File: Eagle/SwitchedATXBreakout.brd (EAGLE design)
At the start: 101.3 x 80 mm, 47 parts, among them K1 ALF1P05, K2 ALF1P05, K3 ALF1P05, K4 ALF1P05, K5 ALF1P05, T1 2N3905, T2 2N3905, T3 2N3905, T4 2N3905, T5 2N3905, X1 22-23-2091, X2 5566-24

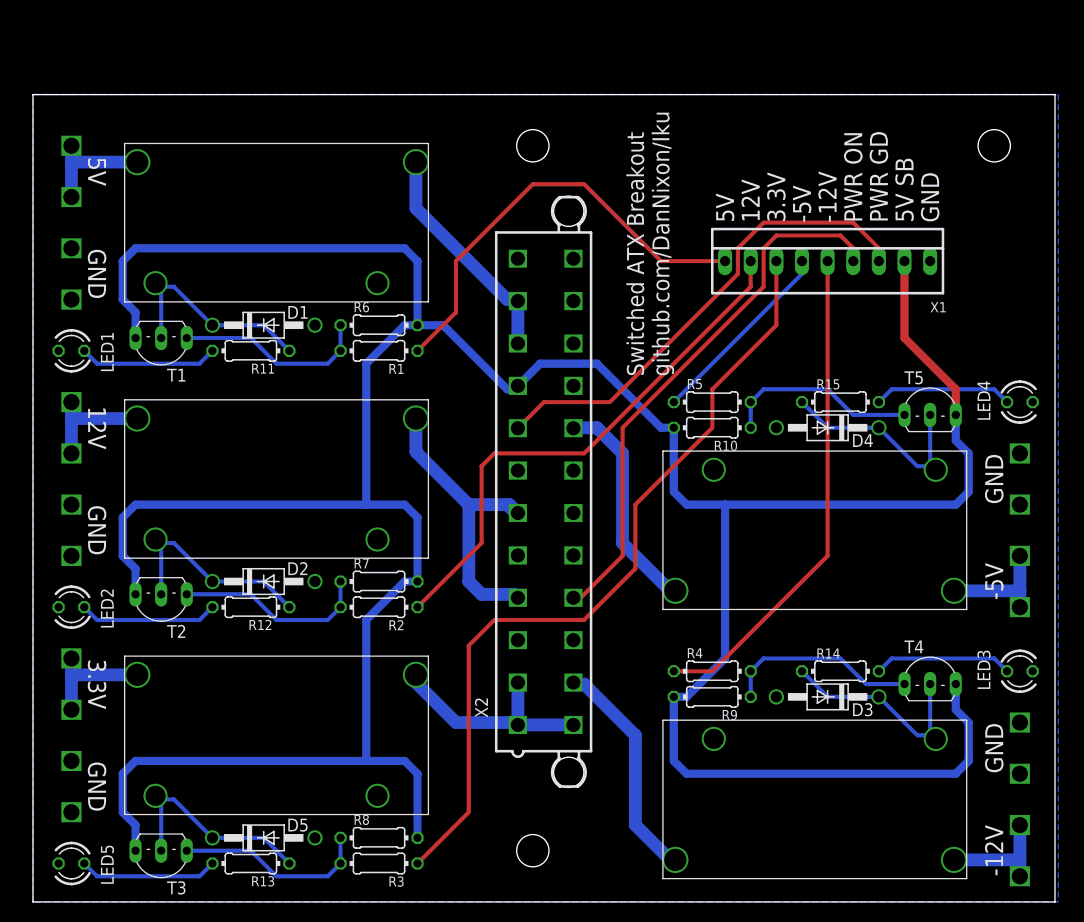
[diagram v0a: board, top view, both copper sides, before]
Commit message: Updated board layout
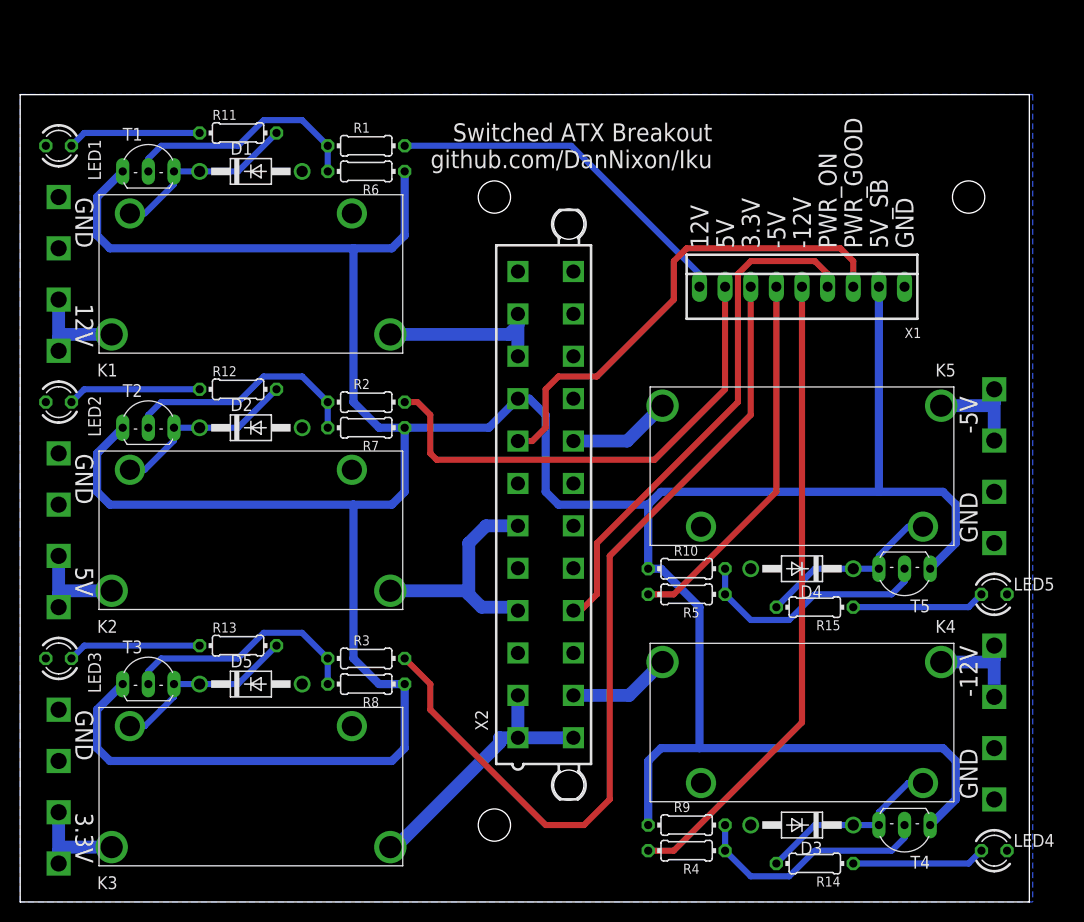
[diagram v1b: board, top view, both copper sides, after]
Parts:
- T1, T2, T3, T4, T5: value 2N3905 -> 2N3906; device transistor:TO92-BCE -> transistor-neu-to92:TO92-EBC
- moved U$8 98.6 mm to (3.81, 67.3)
- moved LED3 95.3 mm to (3.81, 24.1), turned to 180 degrees
- moved U$14 95.3 mm to (3.81, 16.5)
- moved LED5 95.2 mm to (96.5, 30.5), turned to 0 degrees
- moved U$10 91.4 mm to (96.5, 38.1)
- moved U$12 91.4 mm to (96.5, 12.7)
- moved K5 58.5 mm to (77.5, 43.2), turned to 180 degrees
- moved K3 55.9 mm to (22.9, 11.4), turned to 0 degrees
- moved LED4 44.5 mm to (96.5, 5.08)
- moved R11 21.6 mm to (21.6, 76.2)
- moved R13 21.6 mm to (21.6, 25.4)
- moved R12 21.6 mm to (21.6, 50.8)
- moved R15 20.5 mm to (78.7, 29.2)
- moved LED1 20.4 mm to (3.81, 74.9)
- moved R1 20.4 mm to (34.3, 74.9)
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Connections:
- net -12V_OUT: now also K4.NO; no longer K3.NO
- net -5V_OUT: now also K5.NO; no longer K4.NO
- net 3V3_OUT: now also K3.NO; no longer K5.NO
- net N$11: now also K5.COILA; no longer K4.COILA
- net N$12: now also LED3.A; no longer LED5.A
- net N$13: now also LED5.A; no longer LED4.A
- net N$14: now also K3.COILA; no longer K5.COILA
- net N$15: now also LED4.A; no longer LED3.A
- net N$8: now also K4.COILA; no longer K3.COILA
- net PSU_-12V: now also K4.COM; no longer K3.COM
- net PSU_-5V: now also K5.COM; no longer K4.COM
- net PSU_3V3: now also K3.COM; no longer K5.COM
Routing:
- net SW_-5V: track 19.2 -> 37.2 mm
- net SW_-12V: track 49.2 -> 63.7 mm
- net PSU_-12V: track 22.6 -> 10.2 mm
- net PSU_-5V: track 22.0 -> 10.3 mm
- net 5V_SB: track 336.0 -> 344.2 mm
- net SW_12V: track 43.5 -> 35.7 mm
- net SW_3V3: track 79.6 -> 86.3 mm
- net PSU_5V: track 30.5 -> 24.1 mm
- net PSU_12V: track 22.7 -> 17.2 mm
- net PSU_3V3: track 22.3 -> 27.5 mm
- net N$5: track 19.4 -> 24.2 mm
- net N$7: track 19.4 -> 24.2 mm
- net N$2: track 19.4 -> 24.2 mm
- net N$1: track 19.4 -> 24.2 mm
- net N$6: track 19.4 -> 24.2 mm
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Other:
- board size 101.3 x 80 mm -> 100 x 80 mm
- board text added: "5V_SB"
- board text added: "PWR_GOOD"
- board text added: "PWR_ON"
- board text removed: "5V SB"
- board text removed: "PWR GD"
- board text removed: "PWR ON"
